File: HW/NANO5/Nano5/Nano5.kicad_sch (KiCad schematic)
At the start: 52 parts, among them J1 Screw_Terminal_01x03, J10 Screw_Terminal_01x03, J11 Screw_Terminal_01x03, J12 Screw_Terminal_01x02, J2 Screw_Terminal_01x03, J3 Screw_Terminal_01x03, J4 Screw_Terminal_01x03, J5 Screw_Terminal_01x02, J6 Screw_Terminal_01x02, J7 Screw_Terminal_01x02, J8 Screw_Terminal_01x03, J9 Screw_Terminal_01x03, K1 SANYOU_SRD_Form_C, K2 SANYOU_SRD_Form_C, K3 SANYOU_SRD_Form_C, K4 SANYOU_SRD_Form_C, K5 SANYOU_SRD_Form_C, K6 SANYOU_SRD_Form_C, Q1 MMBT3904, Q2 MMBT3904, Q3 MMBT3904, Q4 MMBT3904, Q5 MMBT3904, Q6 MMBT3904

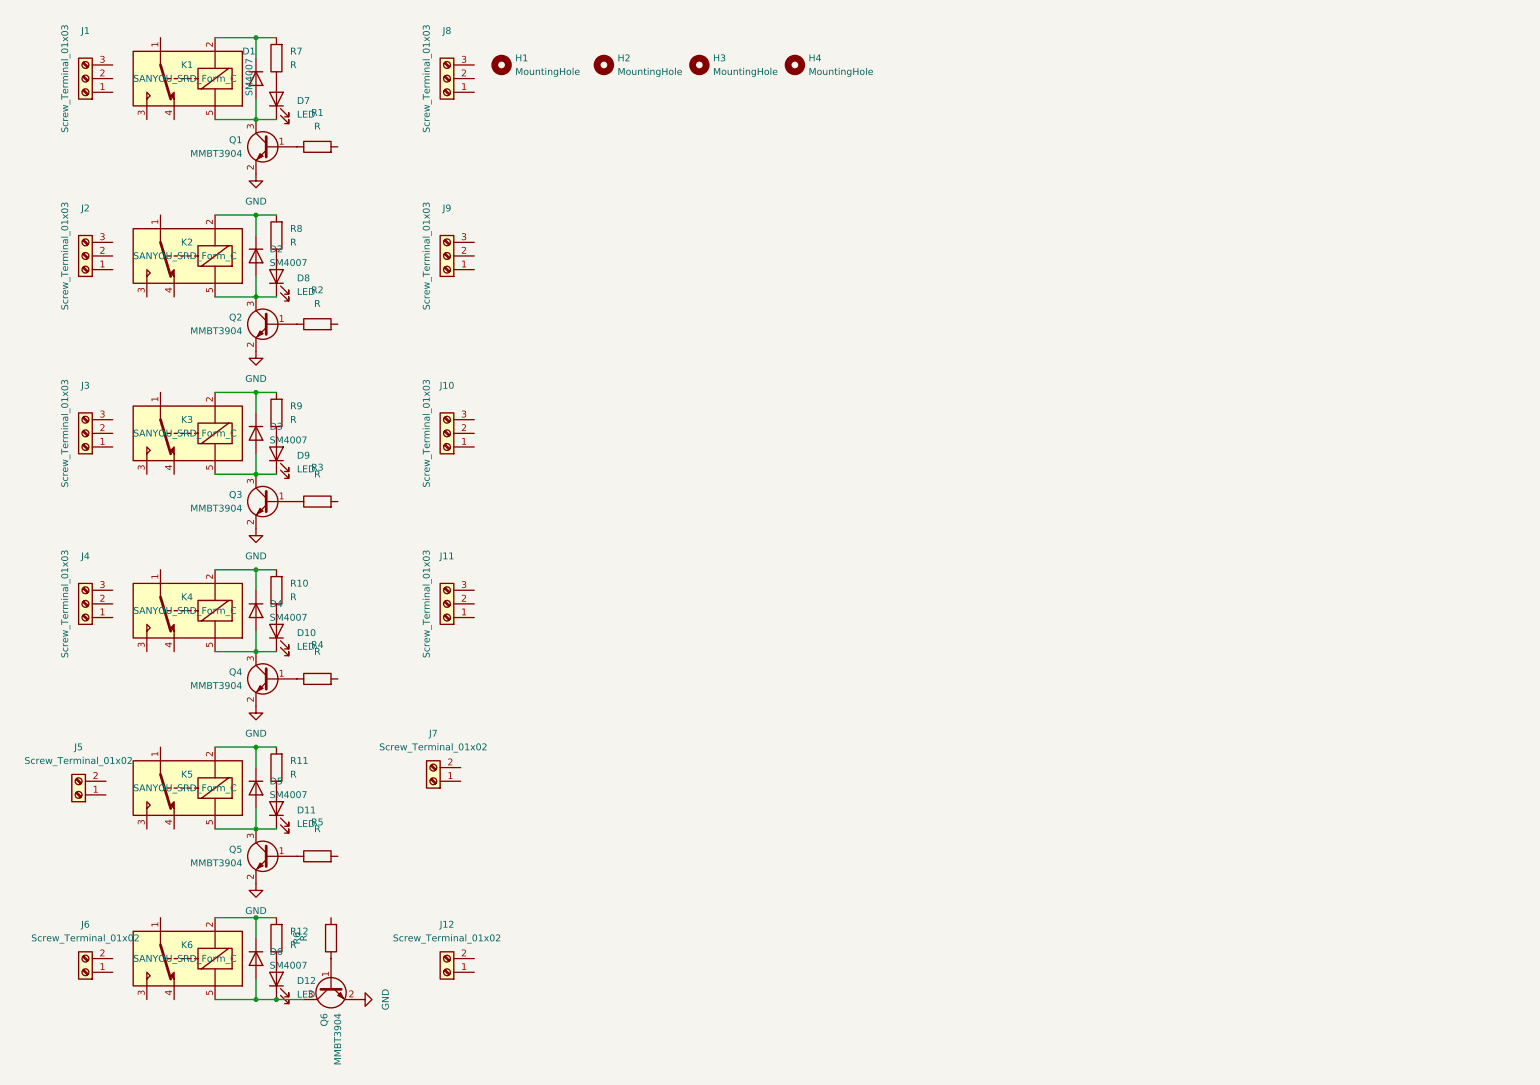
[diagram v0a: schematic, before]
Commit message: add mod 1
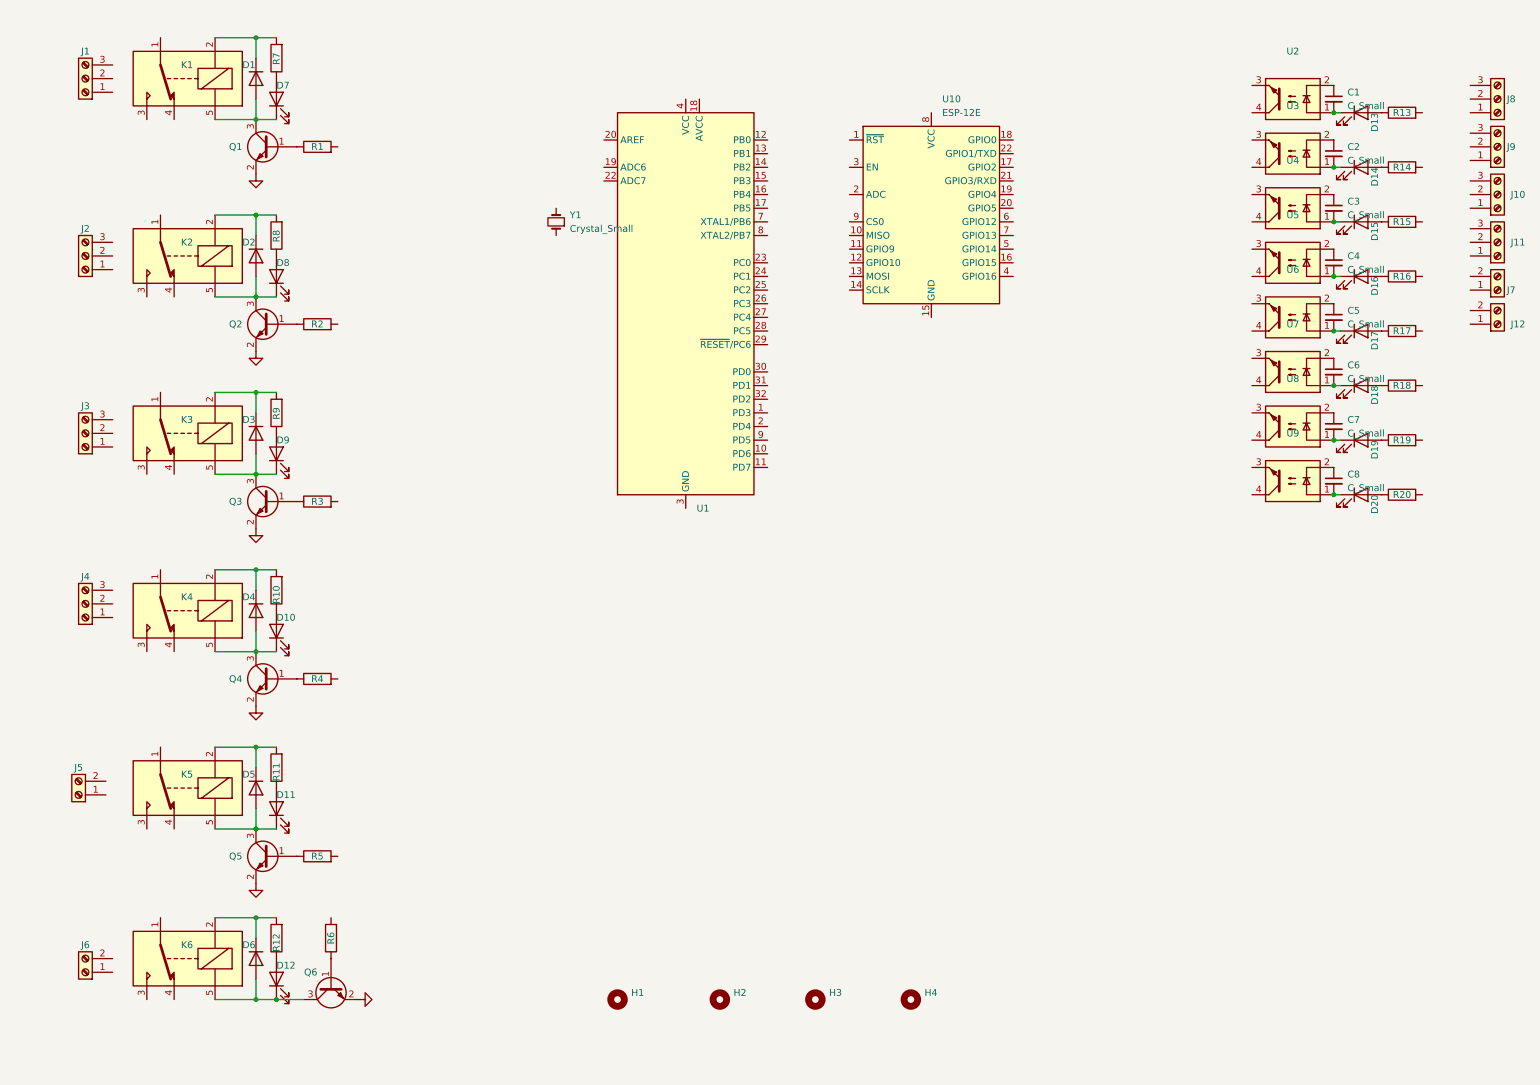
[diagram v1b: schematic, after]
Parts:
- added C1, C2, C3, C4, C5, C6, C7, C8: C_Small, Capacitor_SMD:C_0805_2012Metric, symbol Device:C_Small
- added D13, D14, D15, D16, D17, D18, D19, D20: LED, LED_SMD:LED_0805_2012Metric, symbol Device:LED
- added R13, R14, R15, R16, R17, R18, R19, R20: R, Resistor_SMD:R_0805_2012Metric, symbol Device:R
- added U1: ATmega328P-A, Package_QFP:TQFP-32_7x7mm_P0.8mm, symbol MCU_Microchip_ATmega:ATmega328P-A
- added U10: ESP-12E, RF_Module:ESP-12E, symbol RF_Module:ESP-12E
- added U2, U3, U4, U5, U6, U7, U8, U9: LTV-817S, Package_DIP:SMDIP-4_W9.53mm, symbol Isolator:LTV-817S
- added Y1: Crystal_Small, Crystal:Crystal_SMD_HC49-SD, symbol Device:Crystal_Small
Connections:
- new net: C4.1, U5.2
- new net: C4.2, D16.1 (K), U5.1
- new net: D13.2 (A), R13.1
- new net: C2.2, D14.1 (K), U3.1
- new net: D14.2 (A), R14.1
- new net: C6.1, U7.2
- new net: C6.2, D18.1 (K), U7.1
- new net: C5.2, D17.1 (K), U6.1
- new net: D17.2 (A), R17.1
- new net: D16.2 (A), R16.1
- new net: C2.1, U3.2
- new net: C7.1, U8.2
- new net: C7.2, D19.1 (K), U8.1
- new net: C3.1, U4.2
- new net: C3.2, D15.1 (K), U4.1
- new net: C1.2, D13.1 (K), U2.1
- new net: D15.2 (A), R15.1
- new net: D19.2 (A), R19.1
- new net: C5.1, U6.2
- new net: C8.2, D20.1 (K), U9.1
- new net: D20.2 (A), R20.1
- new net: D18.2 (A), R18.1
- new net: C1.1, U2.2
- new net: C8.1, U9.2
- new net: U1.21 (GND), U1.3 (GND), U1.5 (GND)
- new net: U1.4 (VCC), U1.6 (VCC)
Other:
- moved on the sheet: H1, H2, H3, H4, J10, J11, J12, J7, J8, J9
